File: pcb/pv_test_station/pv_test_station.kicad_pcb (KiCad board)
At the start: 2 copper layers, 16 parts, among them IC1 CT426-HSN830DR, J1 Connector_Panel, J2 Connector_load, J3 Conncector 5V, J4 qwiic, J5 i2c, J6 GPS, K1 AZ576-1A-12DE, Q1 2N7002

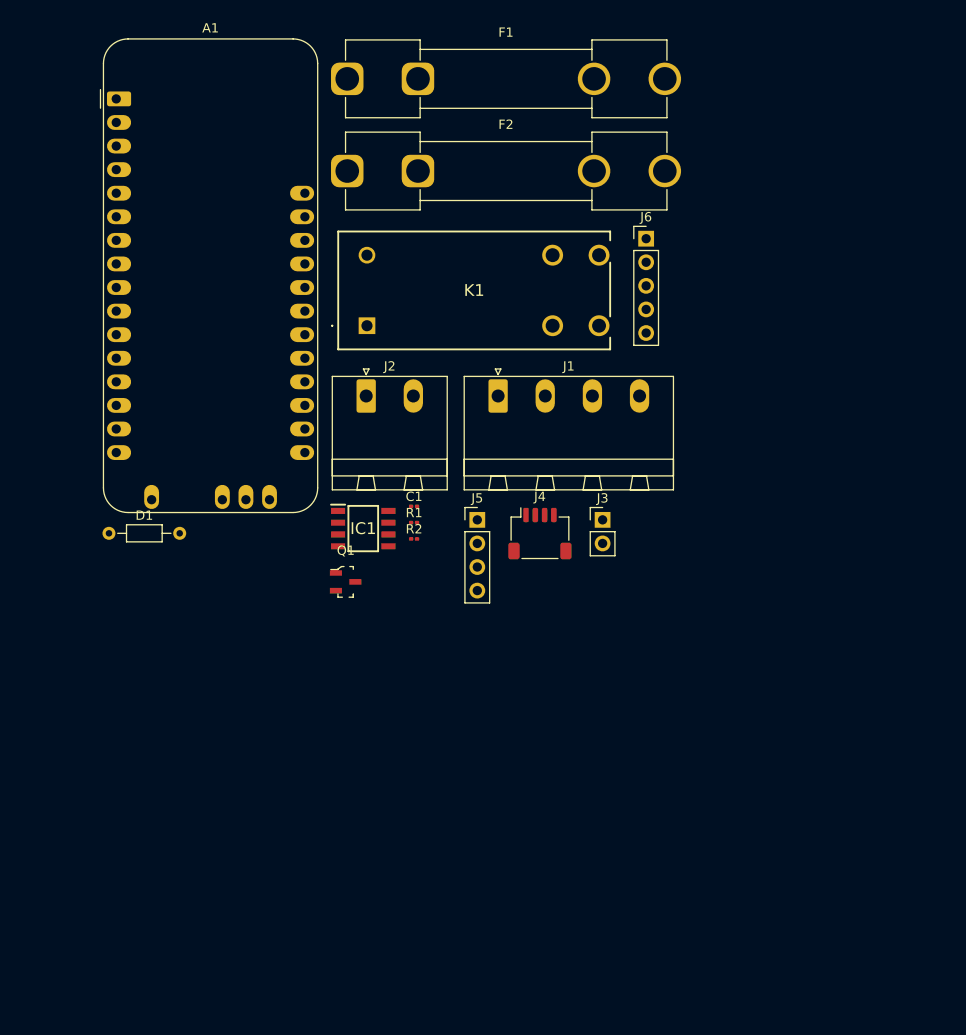
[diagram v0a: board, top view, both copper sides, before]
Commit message: finished pcb
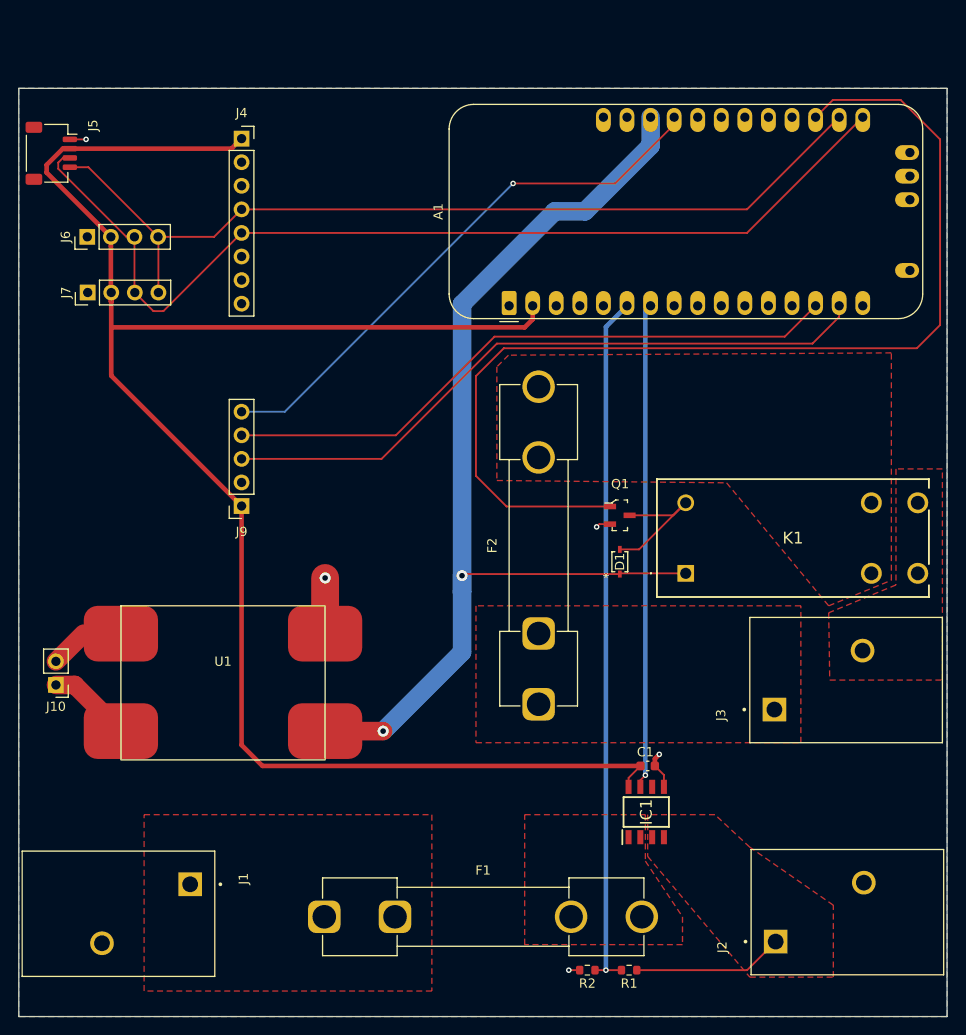
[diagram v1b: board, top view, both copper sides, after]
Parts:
- removed the J3 at (133.4, 99.0)
- added J10: Bat in, Connector_PinHeader_2.54mm:PinHeader_1x02_P2.54mm_Vertical, F.Cu at (74.5, 116.8)
- added J2: Out, digikey-footprints:PHOENIX_1017521, F.Cu at (170.1, 148.0)
- added J4: FRAM, Connector_PinSocket_2.54mm:PinSocket_1x08_P2.54mm_Vertical, F.Cu at (94.5, 57.9)
- added J7: Temp2, Connector_PinHeader_2.54mm:PinHeader_1x04_P2.54mm_Vertical, F.Cu at (77.9, 74.5)
- added U1: ~, digikey-footprints:DCDC, F.Cu at (92.5, 116.8)
- C1: footprint Capacitor_SMD:C_0201_0603Metric -> Capacitor_SMD:C_0603_1608Metric
- D1: footprint Resistor_THT:R_Axial_DIN0204_L3.6mm_D1.6mm_P7.62mm_Horizontal -> digikey-footprints:DIODE_BAR6303WE6327HTSA1_INF
- J1: value Connector_Panel -> In; footprint Connector_Phoenix_MSTB:PhoenixContact_MSTBA_2,5_4-G-5,08_1x04_P5.08mm_Horizontal -> digikey-footprints:PHOENIX_1017521
- J3: renamed from J2; value Connector_load -> load; footprint Connector_Phoenix_MSTB:PhoenixContact_MSTBA_2,5_2-G-5,08_1x02_P5.08mm_Horizontal -> digikey-footprints:PHOENIX_1017521
- J6: renamed from J5; value i2c -> Temp1
- J9: renamed from J6; footprint Connector_PinHeader_2.54mm:PinHeader_1x05_P2.54mm_Vertical -> Connector_PinSocket_2.54mm:PinSocket_1x05_P2.54mm_Vertical
- R1, R2: footprint Resistor_SMD:R_0201_0603Metric -> Resistor_SMD:R_0603_1608Metric
- moved F1 90.3 mm to (103.4, 141.8)
- moved J3 72.4 mm to (170.0, 123.0), turned to 90 degrees
- moved J1 70.9 mm to (70.9, 134.7), turned to -90 degrees
- moved J5 66.7 mm to (74.0, 59.5), turned to -90 degrees
- moved F2 61.0 mm to (126.5, 118.9), turned to 90 degrees
- moved D1 55.1 mm to (135.2, 103.5), turned to 90 degrees
- moved R1 53.5 mm to (136.2, 147.5), turned to 180 degrees
- moved J9 52.2 mm to (94.5, 97.5), turned to 180 degrees
- moved J6 51.9 mm to (77.9, 68.5), turned to 90 degrees
- moved R2 50.1 mm to (131.8, 147.5), turned to 180 degrees
- moved A1 47.8 mm to (123.3, 75.9), turned to 90 degrees
- moved K1 43.5 mm to (142.3, 104.8)
- moved IC1 43.1 mm to (138.1, 130.5), turned to 90 degrees
- moved C1 37.6 mm to (138.2, 125.5), turned to 180 degrees
- moved Q1 30.4 mm to (135.2, 98.5)
- renumbered J4 to J5
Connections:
- net /Relais renamed relais
- A1 pad 2: Net-(A1-3V3) -> +3.3V
- C1 pad 2: Net-(A1-3V3) -> +3.3V
- IC1 pad 8: Net-(A1-3V3) -> +3.3V
- J1 pad 1: /- In -> /+ In
- J1 pad 2: /- In -> GND
- R2 pad 2: /- In -> GND
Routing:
- net +3.3V: track 0.00 -> 206.4 mm
- net /RelaisPin: track 0.00 -> 114.8 mm
- net +5V: track 0.00 -> 112.2 mm, vias 0 -> 2
- net /SDA: track 0.00 -> 107.3 mm
- net /SCL: track 0.00 -> 97.3 mm
- net /V_meter: track 0.00 -> 75.1 mm, vias 0 -> 1
- net /RX: track 0.00 -> 71.9 mm
- net /TX: track 0.00 -> 67.6 mm
- net /PPS: track 0.00 -> 60.2 mm, vias 0 -> 1
- net /A_meter: track 0.00 -> 52.3 mm, vias 0 -> 1
- net /+ Out: track 0.00 -> 16.2 mm
- net Net-(D1-A): track 0.00 -> 15.8 mm
- net GND: track 0.00 -> 14.6 mm, vias 0 -> 5
- net Net-(J10-Pin_1): track 0.00 -> 9.06 mm
- net Net-(J10-Pin_2): track 0.00 -> 8.24 mm
- added copper zone on F.Cu, net /+ In
- added copper zone on F.Cu, net /+ Out
- added copper zone on B.Cu, net GND
- added copper zone on F.Cu, net Net-(IC1-IP+_1)
- added copper zone on F.Cu, net Net-(J3-Pin_2)
- added copper zone on F.Cu, net Net-(K1-COM_1)
- added copper zone on F.Cu, net relais
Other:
- board outline added: 100 x 100 mm
